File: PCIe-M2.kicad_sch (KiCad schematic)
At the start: 10 parts, among them J7 Bus_M.2_Socket_E, M1 M.2 Solder Nut, M2 M.2 Solder Nut, M3 M.2 Solder Nut, M4 M.2 Solder Nut, M5 M.2 Screw, U4 ASEK-32.768KHZ-L-R-T

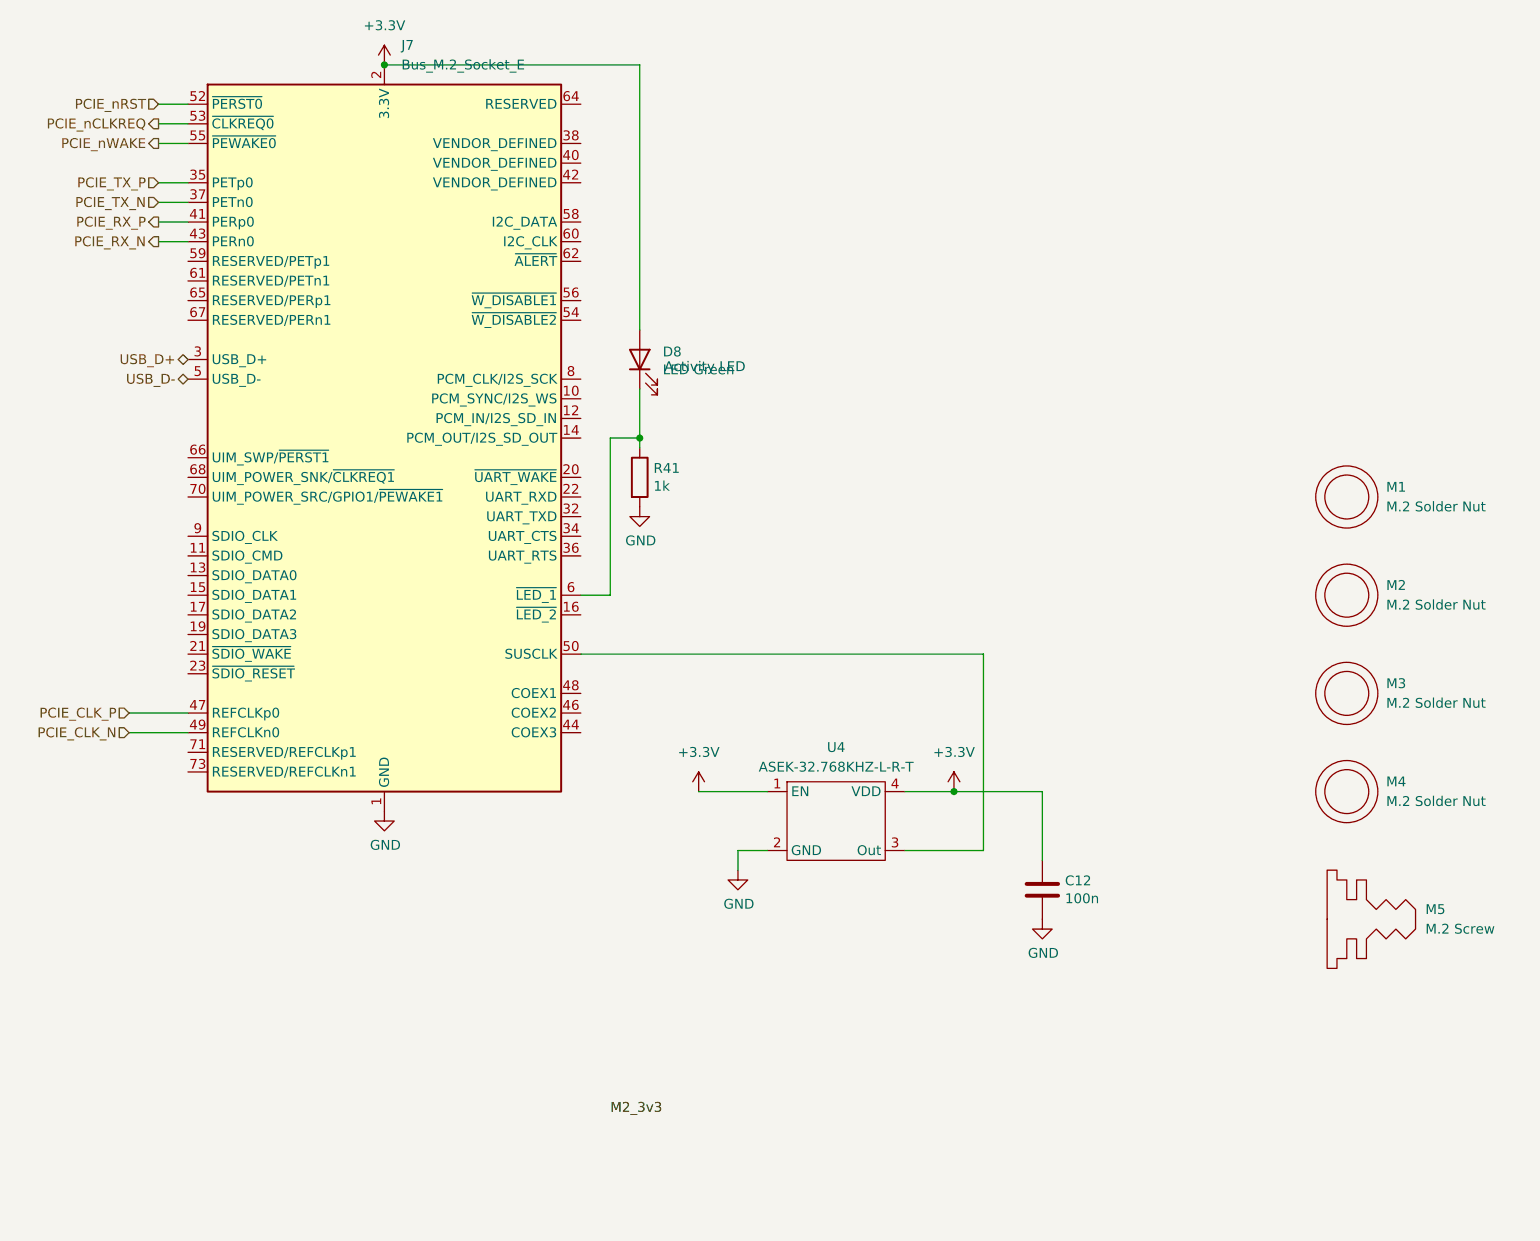
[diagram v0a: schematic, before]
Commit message: change cad data
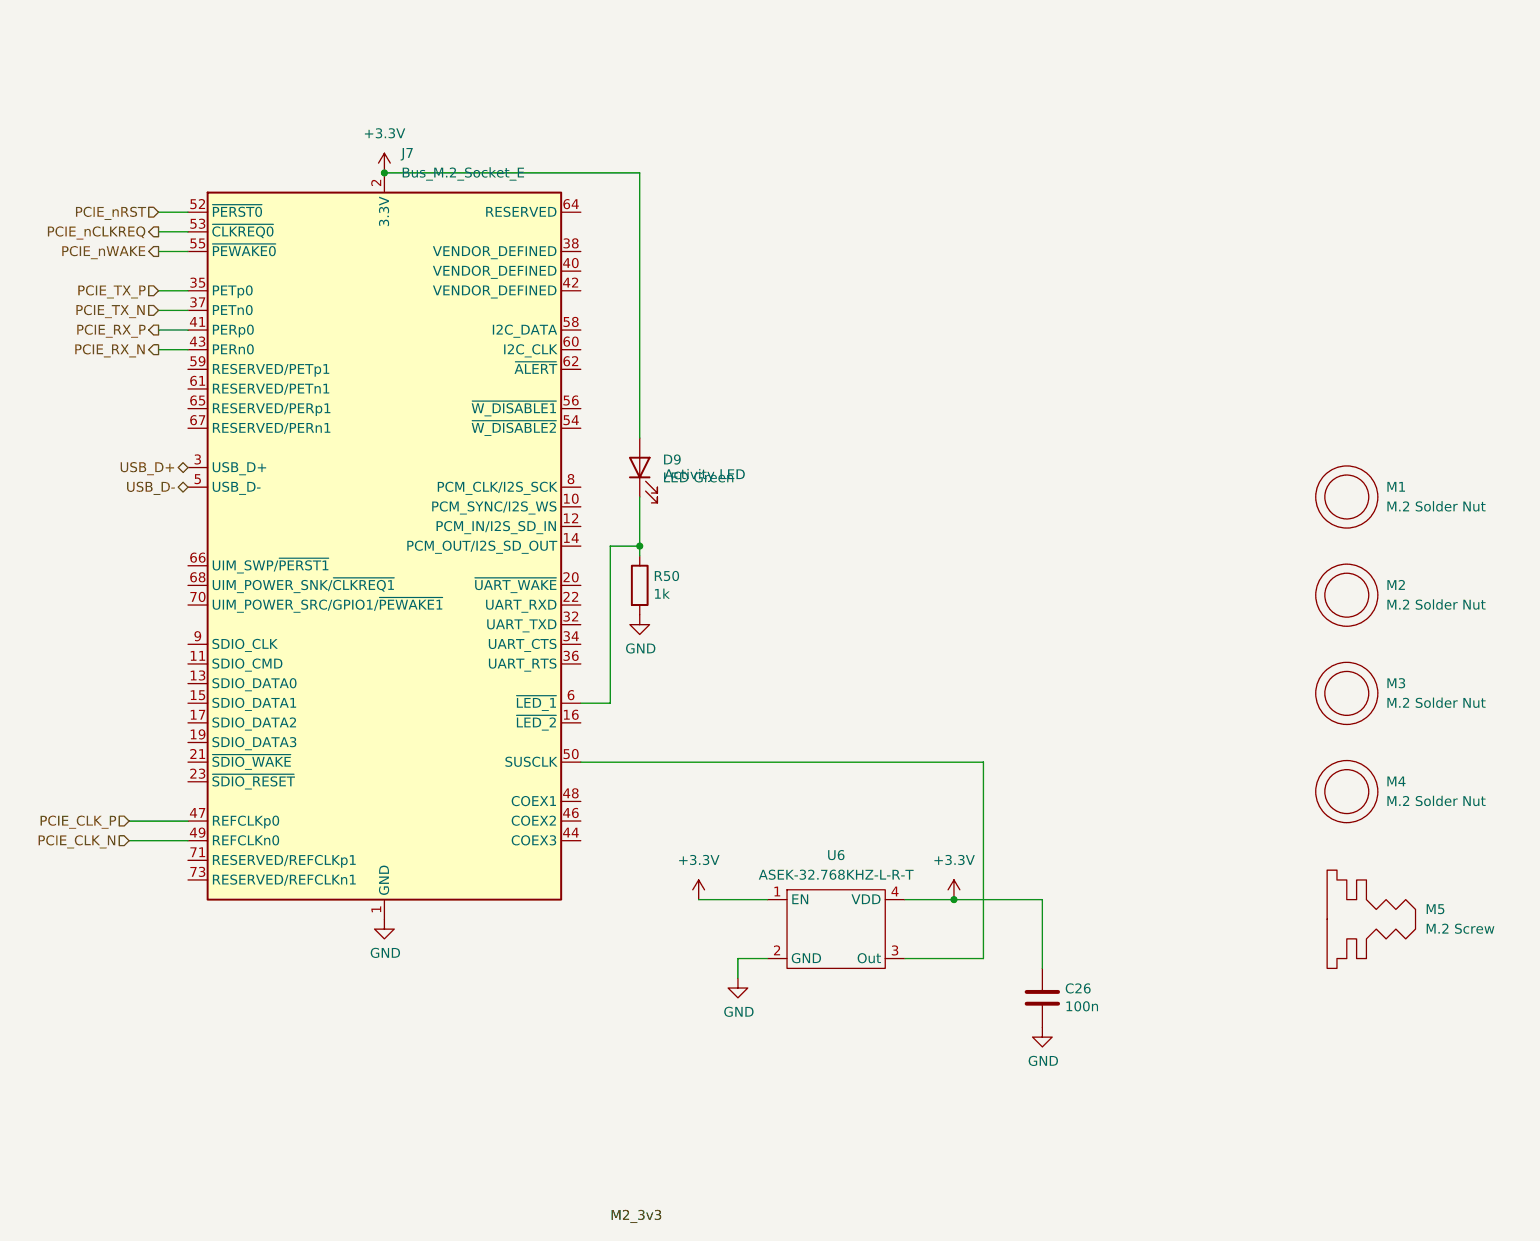
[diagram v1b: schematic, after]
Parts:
- D9: renamed from D8; footprint LED_SMD:LED_0603_1608Metric -> LED_SMD:LED_0603_1608Metric_Pad1.05x0.95mm_HandSolder
- renumbered C12 to C26, R41 to R50, U4 to U6
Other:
- moved on the sheet: C26, D9, J7, R50, U6
